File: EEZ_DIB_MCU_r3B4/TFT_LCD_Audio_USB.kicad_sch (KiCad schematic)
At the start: 36 parts, among them IC11 TPS2051BDBVR, IC12 TPS61169DCKR, IC13 TPD4E001DRLR, IC14 TSC2007IPW, J2 67803-8020, Q1 N.C., Q2 2N7002

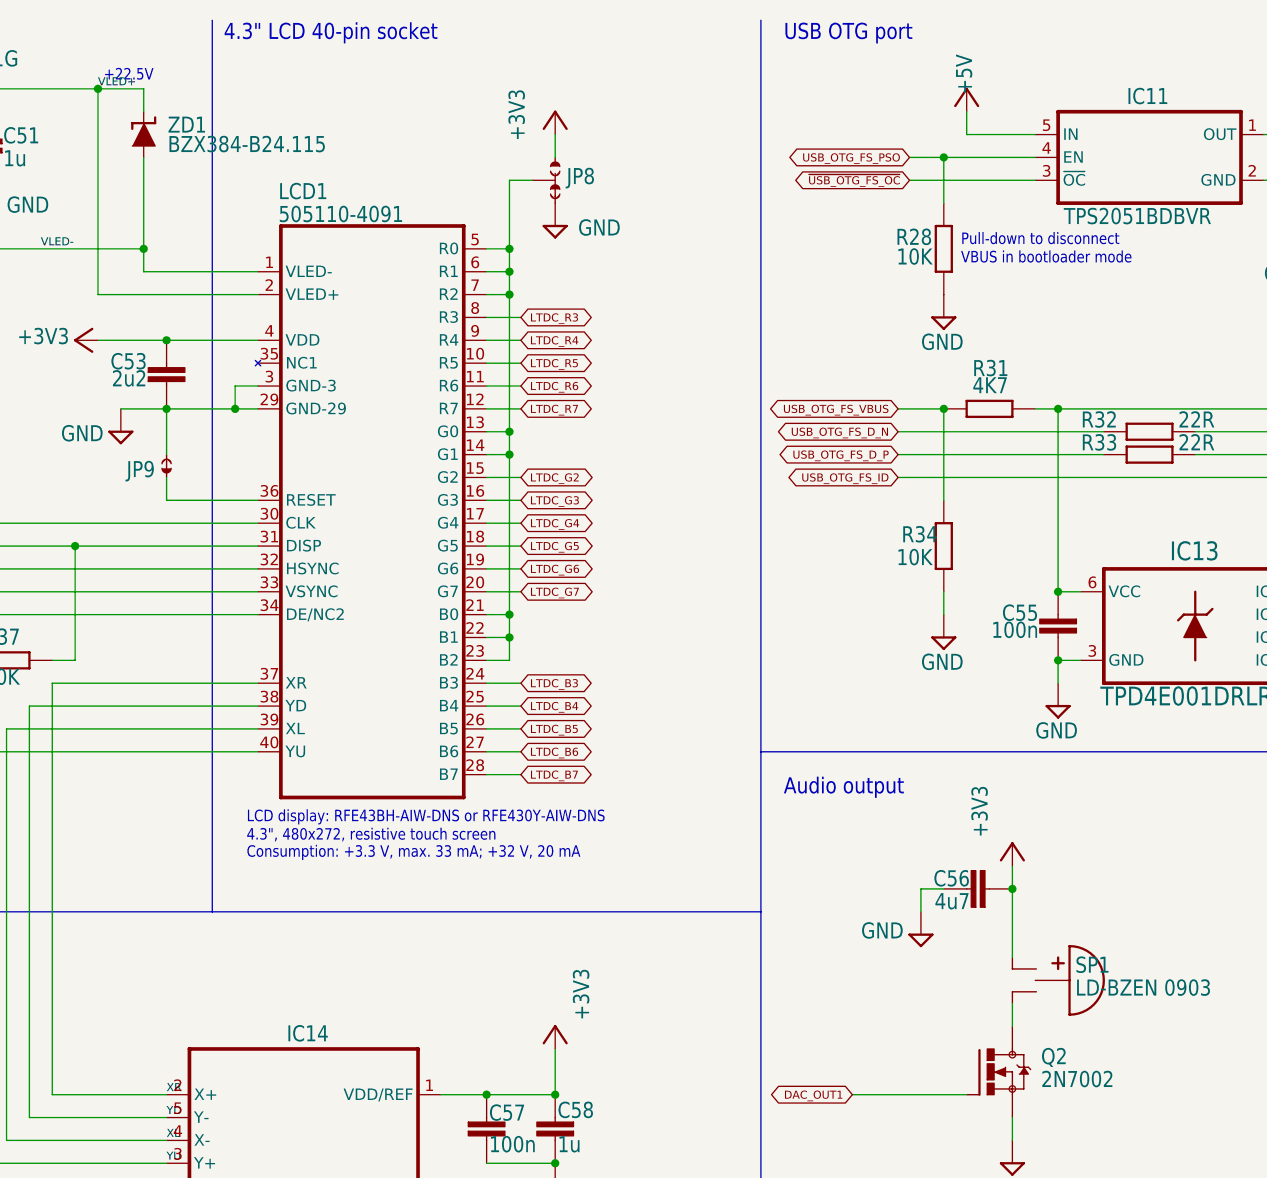
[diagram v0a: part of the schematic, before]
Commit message: Switching MCU to KiCad 7 - moving MCU and SDRAM from board
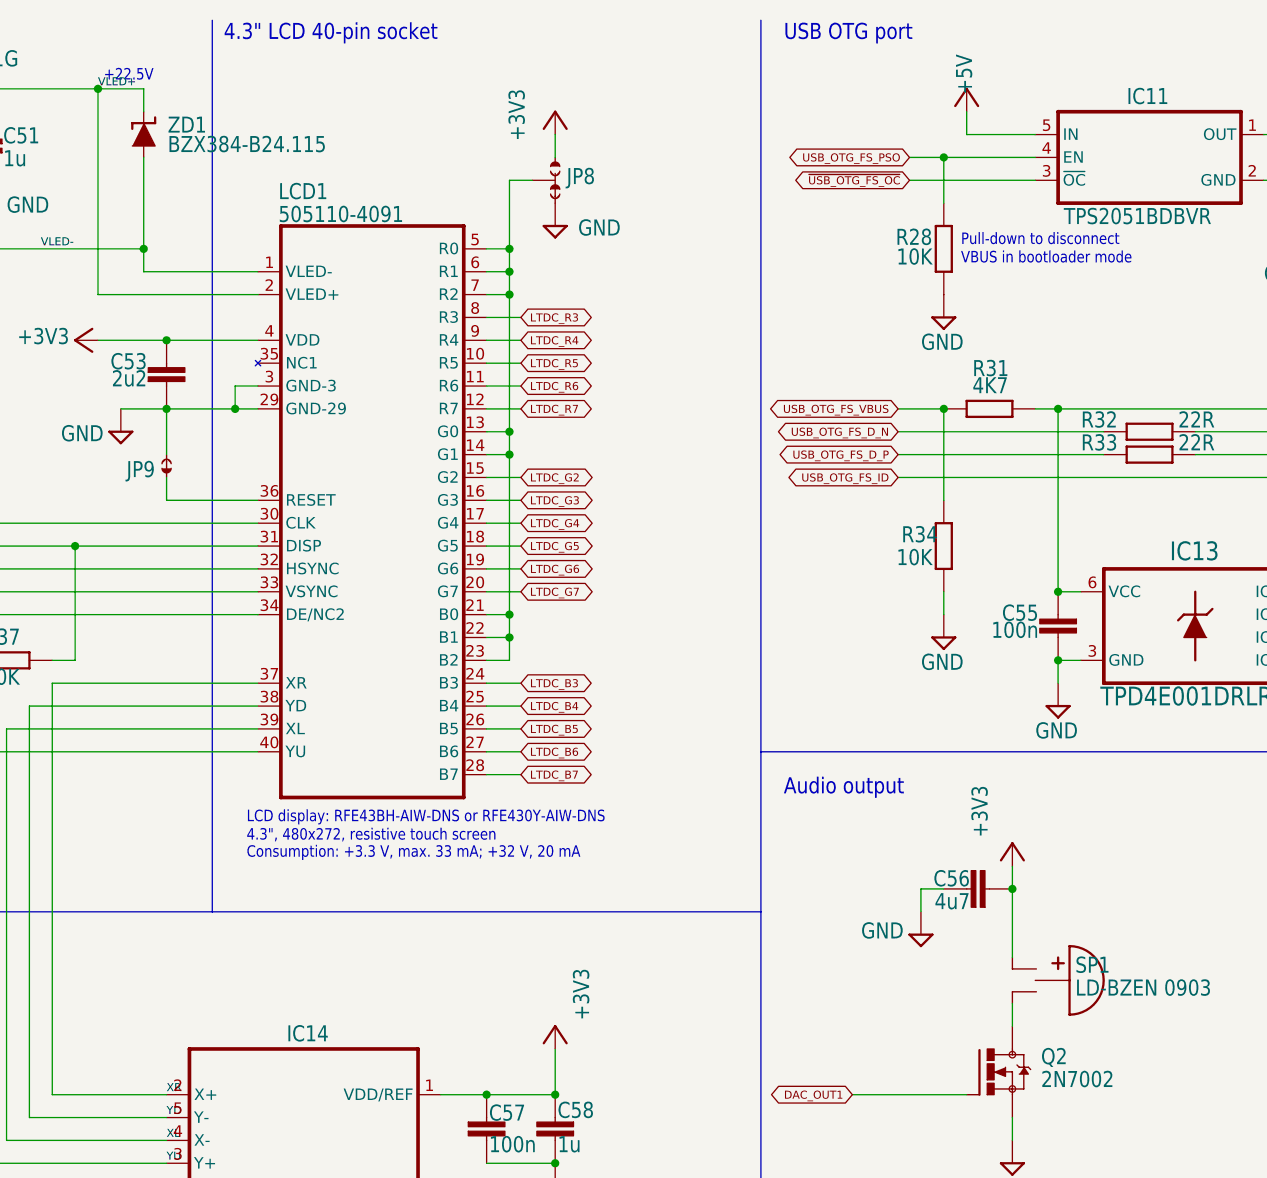
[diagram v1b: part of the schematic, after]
